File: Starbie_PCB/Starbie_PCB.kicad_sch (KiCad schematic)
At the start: 7 parts, among them J1 Conn_01x04_Pin, J2 Conn_01x08_Pin, SW1 SW_Push, SW2 SW_Push, U1 DHT11, U2 XIAO-ESP32-C3-SMD

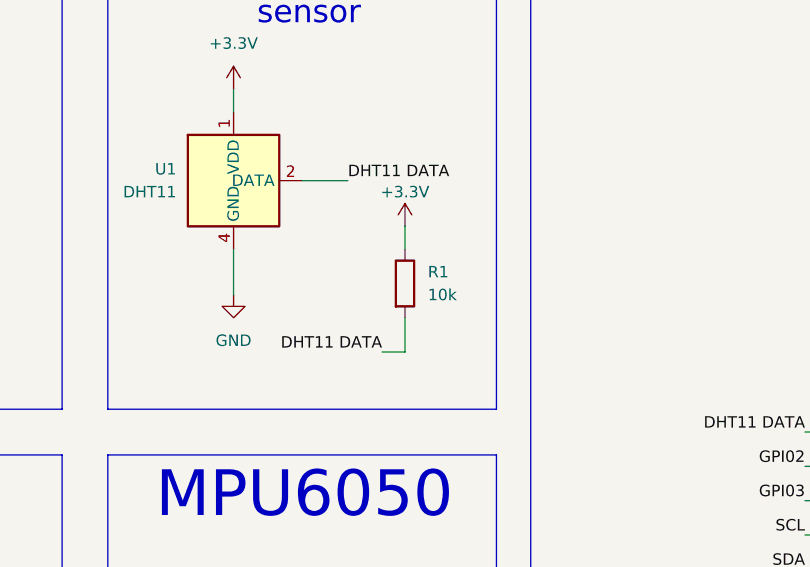
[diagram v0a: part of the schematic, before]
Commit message: Day 2
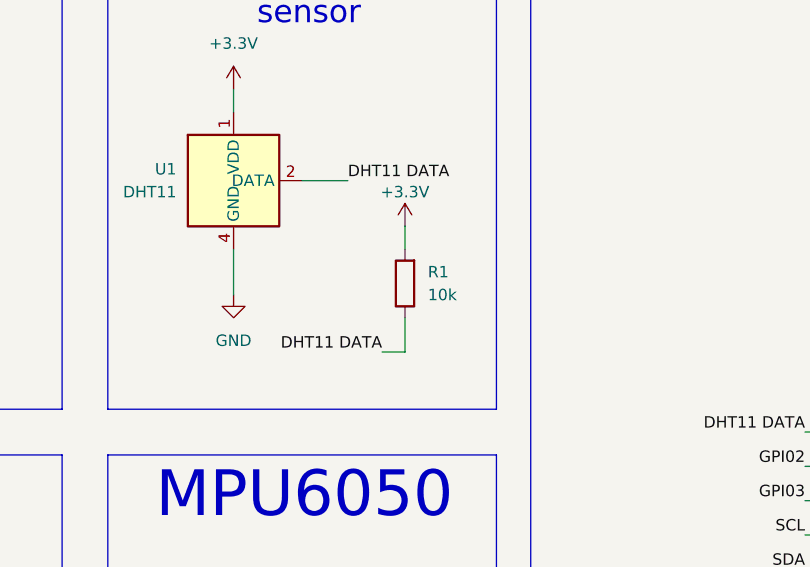
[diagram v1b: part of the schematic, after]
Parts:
- J1: footprint (none) -> Imported Parts:Display_128x64_096_I2C
- J2: footprint (none) -> Connector_PinHeader_2.54mm:PinHeader_1x08_P2.54mm_Vertical
- R1: footprint Package_DIP:DIP-8_W7.62mm -> Resistor_THT:R_Axial_DIN0204_L3.6mm_D1.6mm_P7.62mm_Horizontal
- SW1, SW2: footprint (none) -> Button_Switch_Keyboard:SW_Cherry_MX_1.00u_PCB
- U2: footprint Seeed_Studio_XIAO_Series:XIAO-ESP32-C3-SMD -> Imported Parts:XIAO-ESP32-C6-DIP
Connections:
- net +3.3V: now also R1.2; no longer R1.1
- net DHT11 DATA: now also R1.1; no longer R1.2
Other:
- moved on the sheet: R1
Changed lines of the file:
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@@
 			)
 		)
-		(property "Footprint" ""
+		(property "Footprint" "Imported Parts:Display_128x64_096_I2C"
 			(at 40.64 113.03 0)
 			(hide yes)
@@
 			)
 		)
-		(property "Footprint" "Seeed_Studio_XIAO_Series:XIAO-ESP32-C3-SMD"
+		(property "Footprint" "Imported Parts:XIAO-ESP32-C6-DIP"
 			(at 137.922 104.394 0)
 			(hide yes)
@@
 	(symbol
 		(lib_id "Device:R")
-		(at 106.68 59.69 0)
+		(at 106.68 59.69 180)
 		(unit 1)
 		(body_style 1)
@@
 					(size 1.27 1.27)
 				)
-				(justify left)
+				(justify right)
 			)
 		)
@@
 					(size 1.27 1.27)
 				)
-				(justify left)
-			)
-		)
-		(property "Footprint" "Package_DIP:DIP-8_W7.62mm"
-			(at 104.902 59.69 90)
+				(justify right)
+			)
+		)
+		(property "Footprint" "Resistor_THT:R_Axial_DIN0204_L3.6mm_D1.6mm_P7.62mm_Horizontal"
+			(at 108.458 59.69 90)
 			(hide yes)
 			(show_name no)
@@
 			)
 		)
-		(property "Footprint" ""
+		(property "Footprint" "Connector_PinHeader_2.54mm:PinHeader_1x08_P2.54mm_Vertical"
 			(at 83.82 114.3 0)
 			(hide yes)
@@
 			)
 		)
-		(property "Footprint" ""
+		(property "Footprint" "Button_Switch_Keyboard:SW_Cherry_MX_1.00u_PCB"
 			(at 43.18 38.1 0)
 			(hide yes)
@@
 			)
 		)
-		(property "Footprint" ""
+		(property "Footprint" "Button_Switch_Keyboard:SW_Cherry_MX_1.00u_PCB"
 			(at 43.18 57.15 0)
 			(hide yes)
